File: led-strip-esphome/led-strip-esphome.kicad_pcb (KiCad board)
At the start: 2 copper layers, 47 parts, among them Q1 FS8205A_C2830320, SW1 TS-1002S-04526C, U1 TP4056_C725790, U2 BL8072COTR33, U3 AI-WB2-12F, U4 LGS63042, U5 DW01A, U6 XDM254-1-02-W-8.5-G0

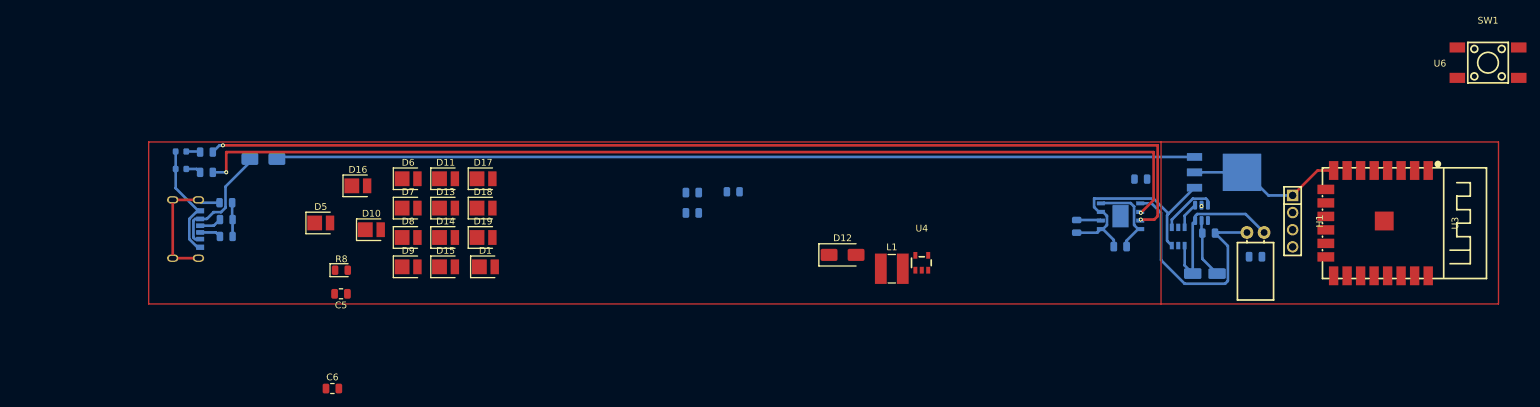
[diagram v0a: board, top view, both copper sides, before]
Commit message: finishing
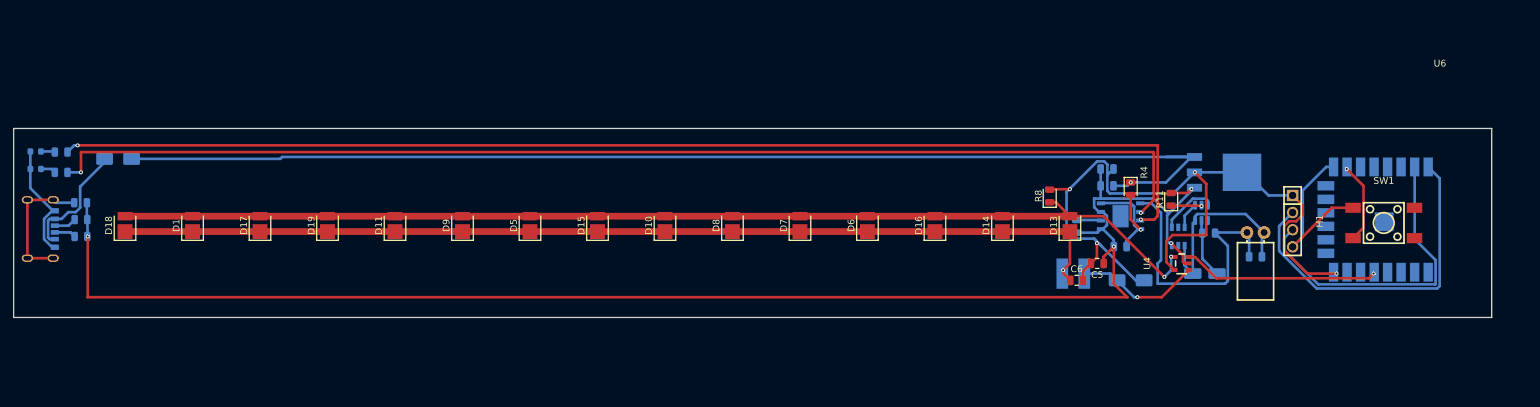
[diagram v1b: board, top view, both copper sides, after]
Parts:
- D12, L1, U3: moved to B.Cu
- R11, R4: moved to F.Cu
- moved C5 112.1 mm to (176.1, 53.0)
- moved C6 111.4 mm to (173.0, 55.5)
- moved R8 105.5 mm to (169.0, 43.0), turned to 90 degrees
- moved D13 92.5 mm to (172.0, 47.4), turned to 90 degrees
- moved D16 85.7 mm to (152.0, 47.4), turned to 90 degrees
- moved D14 82.5 mm to (162.0, 47.4), turned to 90 degrees
- moved D6 68.4 mm to (142.0, 47.4), turned to 90 degrees
- moved C3 61.6 mm to (177.5, 41.5), turned to 180 degrees
- moved C4 61.5 mm to (177.5, 39.0), turned to 180 degrees
- moved R4 58.9 mm to (181.0, 41.9), turned to -90 degrees
- moved D7 58.1 mm to (132.0, 47.4), turned to 90 degrees
- moved D18 53.1 mm to (32.0, 47.4), turned to 90 degrees
- moved D8 48.1 mm to (122.0, 47.4), turned to 90 degrees
- moved D1 43.8 mm to (42.0, 47.4), turned to 90 degrees
- moved D10 43.5 mm to (112.0, 47.4), turned to 90 degrees
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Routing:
- net GND: track 41.2 -> 254.5 mm, vias 0 -> 4
- net Net-(D1-A): track 0.00 -> 165.0 mm, vias 0 -> 2
- net Net-(D1-K): track 0.00 -> 148.1 mm, vias 0 -> 1
- net VCC: track 23.6 -> 115.9 mm, vias 0 -> 4
- net TX: track 0.00 -> 51.1 mm
- net RX: track 0.00 -> 46.8 mm
- net /3V~4.2V Out: track 135.2 -> 175.6 mm, vias 0 -> 1
- net Net-(U3-IO14): track 0.00 -> 28.9 mm, vias 0 -> 1
- net Net-(U1-~{STDBY}): track 152.2 -> 173.7 mm
- net Net-(U1-~{CHRG}): track 153.6 -> 175.2 mm
- net Net-(D12-A): track 0.00 -> 18.7 mm, vias 0 -> 1
- net Net-(U3-IO4): track 0.00 -> 11.9 mm, vias 0 -> 1
- net +: track 35.1 -> 41.6 mm
- net Net-(D2-A): track 30.0 -> 36.0 mm, vias 0 -> 1
- net Net-(U5-CS): track 0.00 -> 4.53 mm
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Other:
- board outline added: 219 x 28 mm
